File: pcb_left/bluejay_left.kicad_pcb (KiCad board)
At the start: 2 copper layers, 17.2 x 1.3 mm, 72 parts, among them J1 SJ-43514, U1 ATmega328P-PU, Y1 16MHz

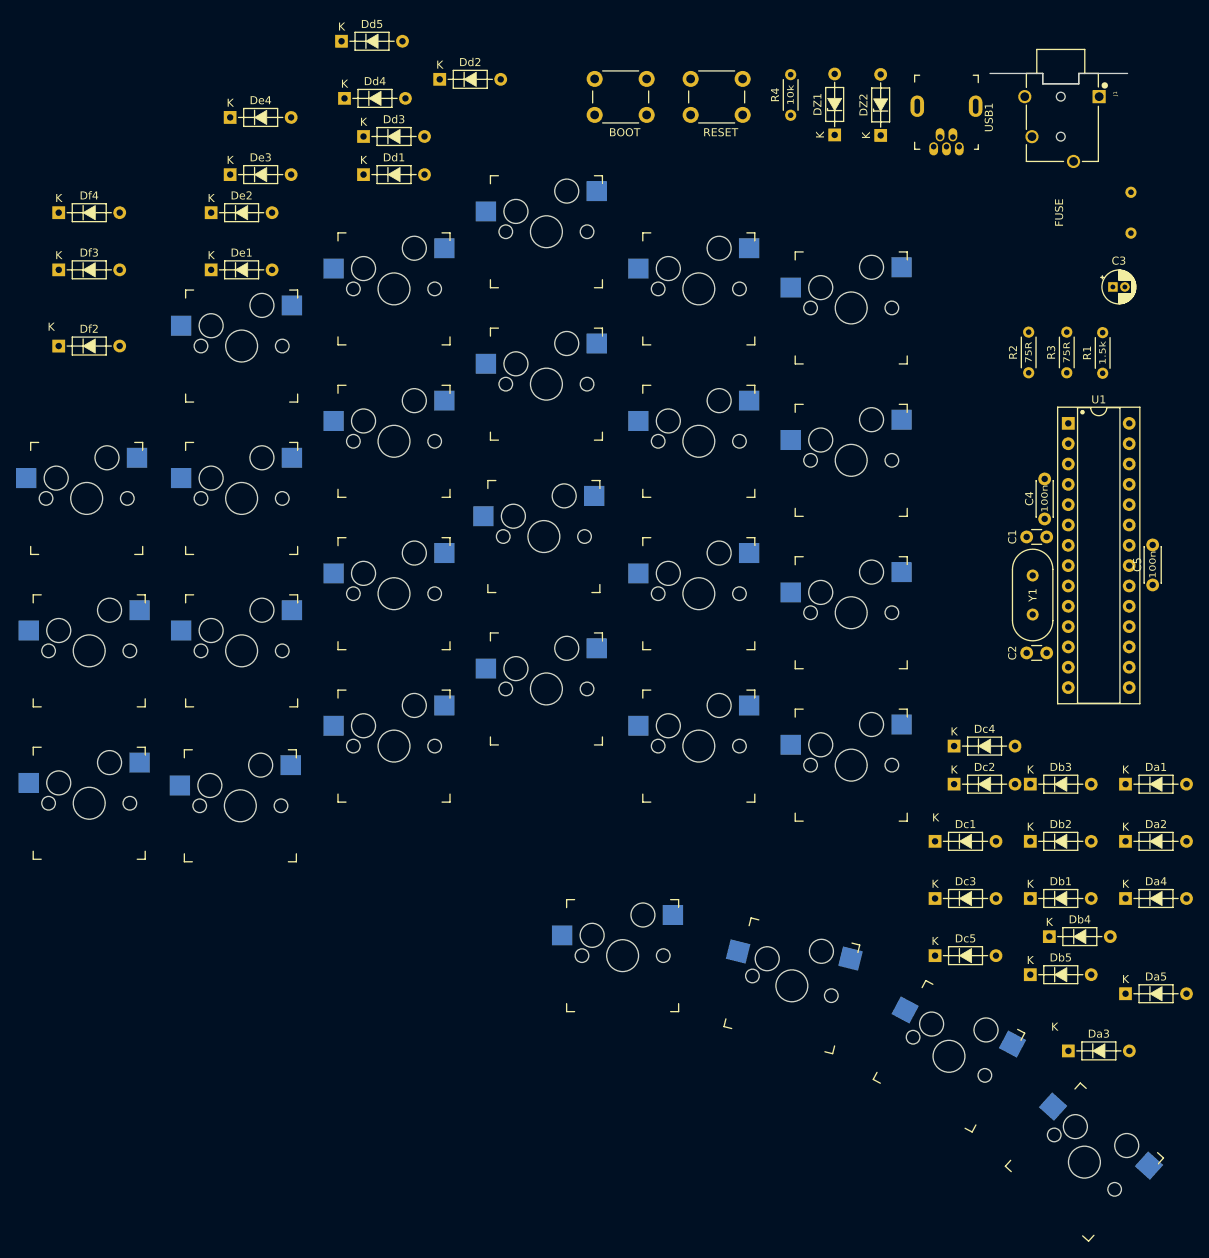
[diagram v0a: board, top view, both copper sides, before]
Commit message: Further work on pcbs
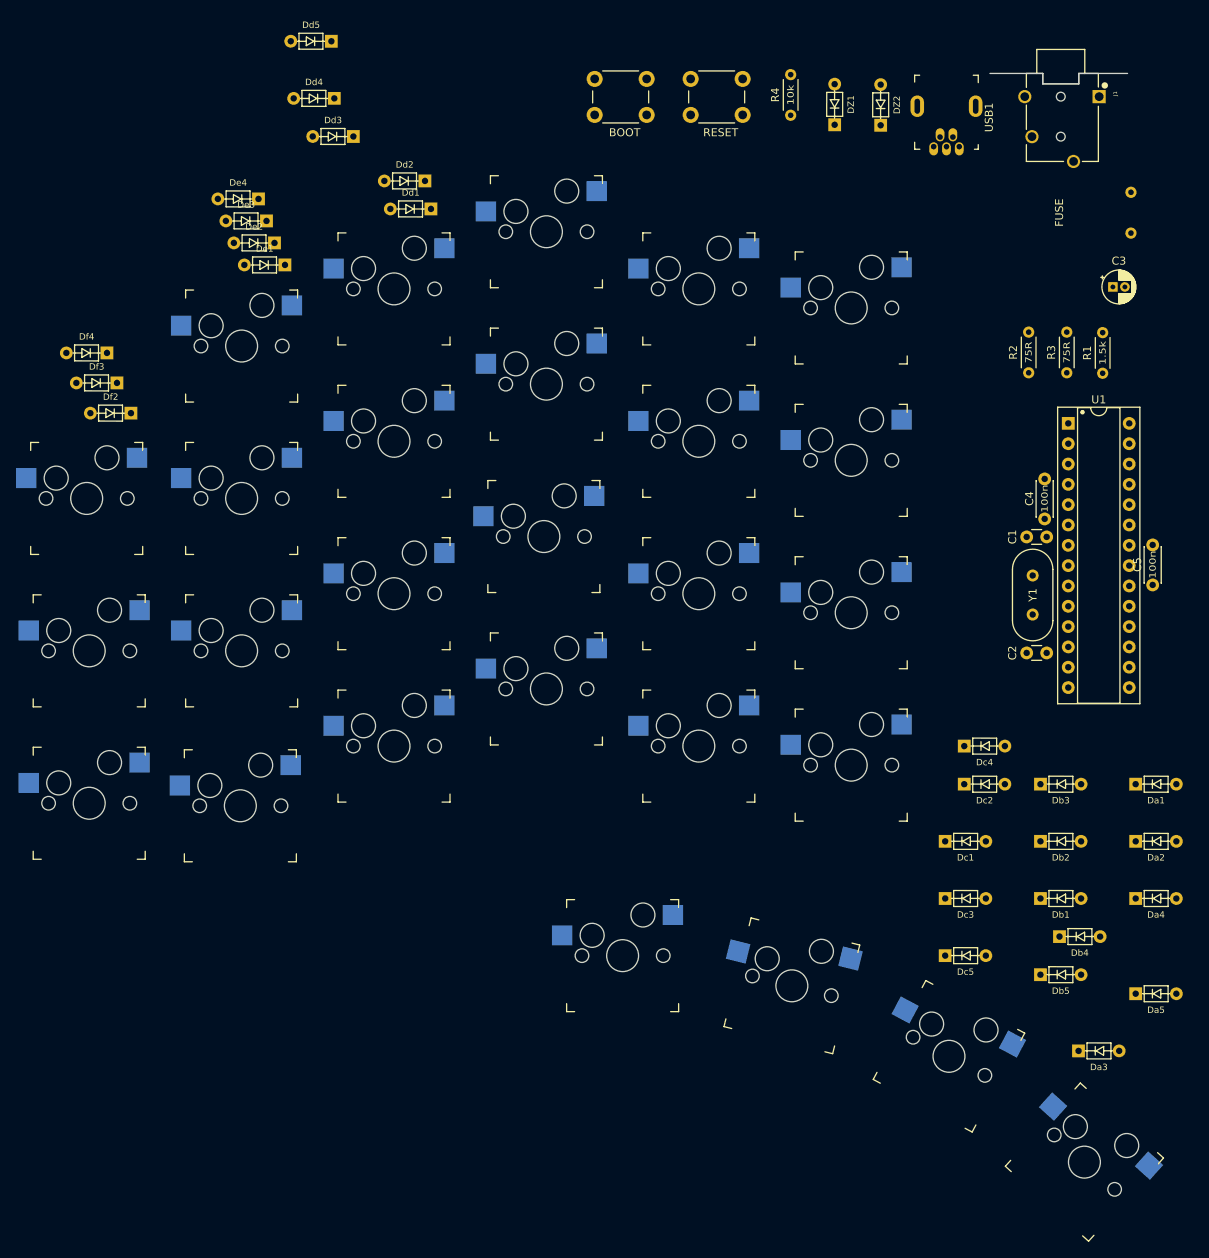
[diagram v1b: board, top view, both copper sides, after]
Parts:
- DZ1, DZ2: footprint Diode_THT_AKL:D_DO-35_SOD27_P7.62mm_Horizontal_Zener -> BlueJay footprints:D_DO-35_SOD27_P5.08mm_Horizontal
- Da1, Da2, Da3, Da4, Da5, Db1, Db2, Db3, Db4, Db5, Dc1, Dc2, Dc3, Dc4, Dc5, Dd1, Dd2, Dd3, Dd4, Dd5, De1, De2, De3, De4, Df2, Df3, Df4: footprint Diode_THT_AKL:D_DO-35_SOD27_P7.62mm_Horizontal -> BlueJay footprints:D_DO-35_SOD27_P5.08mm_Horizontal
- moved Df4 19.0 mm to (77.3, 53.2), turned to 180 degrees
- moved Df3 16.5 mm to (78.6, 57.0), turned to 180 degrees
- moved Df2 13.3 mm to (80.3, 60.8), turned to 180 degrees
- moved Dd2 12.7 mm to (117.1, 31.8), turned to 180 degrees
- moved De4 11.3 mm to (96.2, 34.0), turned to 180 degrees
- moved Dd1 10.6 mm to (117.8, 35.2), turned to 180 degrees
- moved De1 10.5 mm to (99.6, 42.2), turned to 180 degrees
- moved De2 9.94 mm to (98.2, 39.5), turned to 180 degrees
- moved De3 8.21 mm to (97.2, 36.8), turned to 180 degrees
- turned Dd3 to 180 degrees
- turned Dd4 to 180 degrees
- turned Dd5 to 180 degrees
